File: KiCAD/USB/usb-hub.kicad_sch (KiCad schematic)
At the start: 3 parts, among them J1 Conn_01x10_Pin, J2 Conn_01x10_Pin, J3 Conn_01x04_Socket

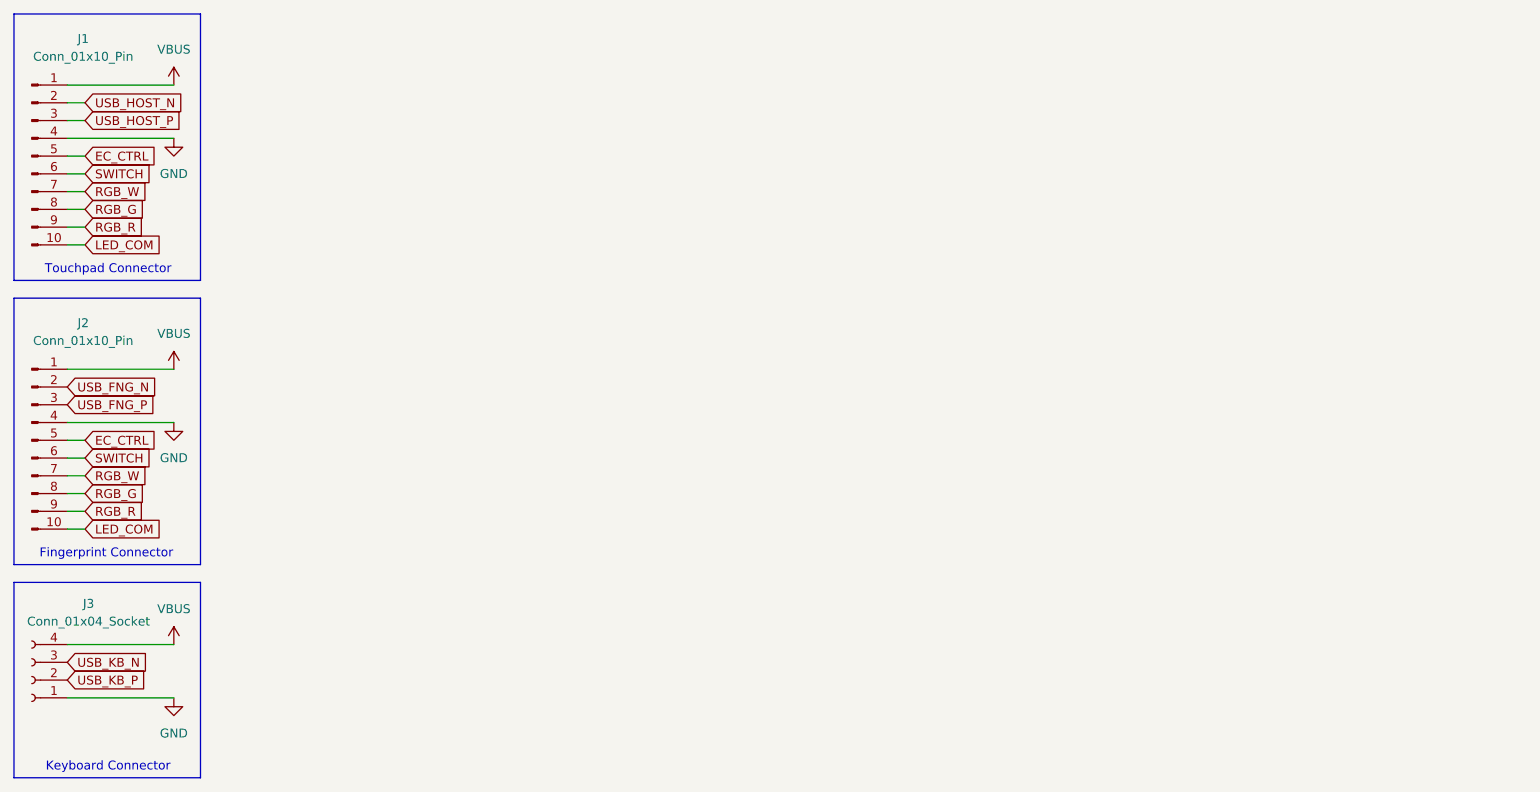
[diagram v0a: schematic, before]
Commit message: mmmm... usb hub controller...
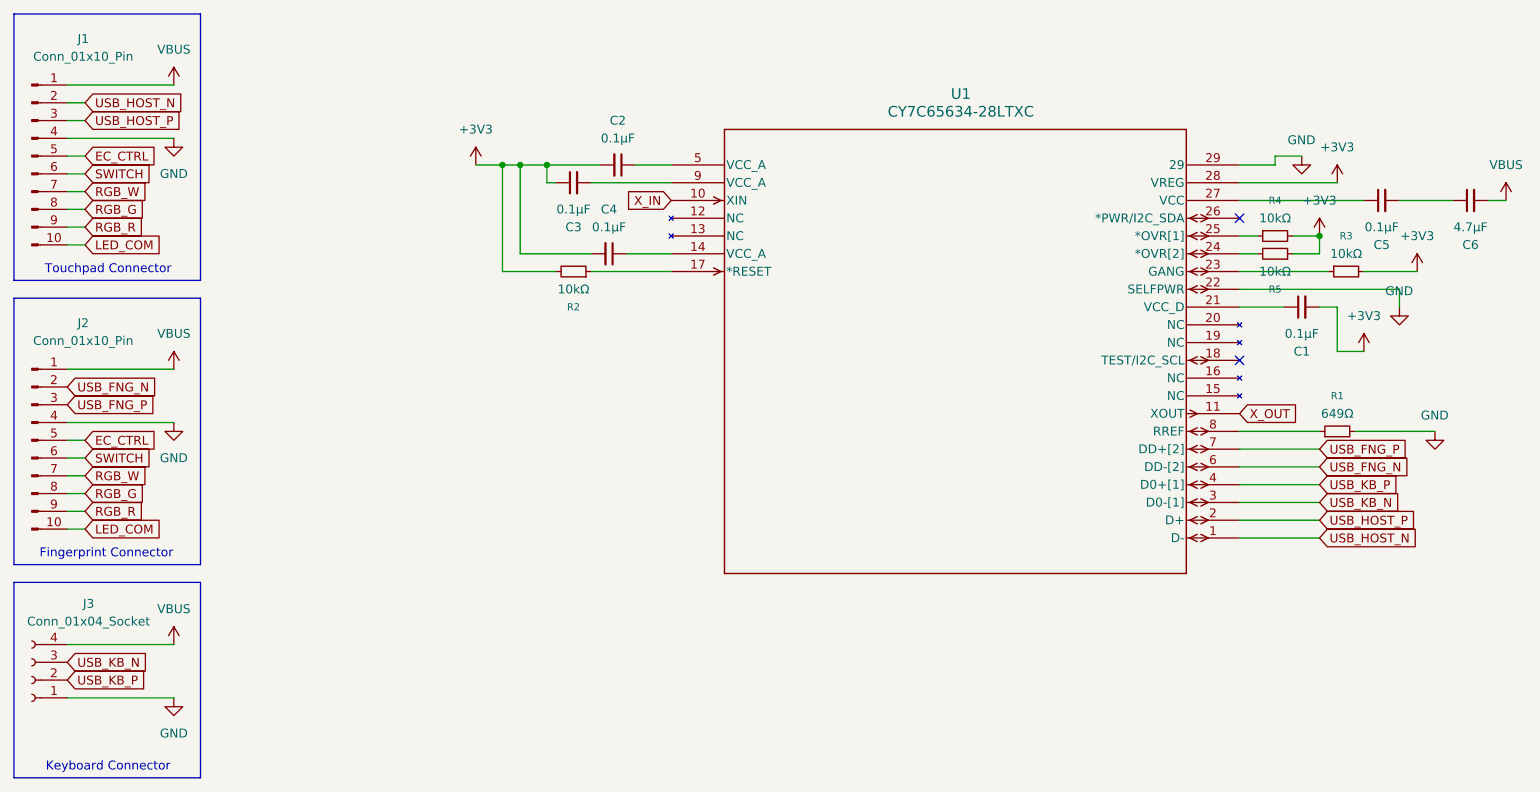
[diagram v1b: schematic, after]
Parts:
- added C1, C2, C3, C4, C5: 0.1μF, symbol Device:C_Small
- added C6: 4.7μF, symbol Device:C_Small
- added R1: 649Ω, symbol Device:R_Small
- added R2, R3, R4, R5: 10kΩ, symbol Device:R_Small
- added U1: CY7C65634-28LTXC, QFN-28, symbol 2025-09-11_12-45-01:CY7C65634-28LTXC
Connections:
- net GND: now also R1.2, U1.22 (SELFPWR), U1.29
- net USB_FNG_N: now also U1.6 (DD-[2])
- net USB_FNG_P: now also U1.7 (DD+[2])
- net USB_HOST_N: now also U1.1 (D-)
- net USB_HOST_P: now also U1.2 (D+)
- net USB_KB_N: now also U1.3 (D0-[1])
- net USB_KB_P: now also U1.4 (D0+[1])
- net VBUS: now also C6.2
- new net: R3.1, U1.23 (GANG)
- new net: C3.2, U1.9 (VCC_A)
- new net: R1.1, U1.8 (RREF)
- new net: C2.1, U1.5 (VCC_A)
- new net: R5.2, U1.24 (*OVR[2])
- new net: R4.1, U1.25 (*OVR[1])
- new net: C5.2, C6.1
- new net: C5.1, U1.27 (VCC)
- new net: R2.1, U1.17 (*RESET)
- new net: C4.1, U1.14 (VCC_A)
- new net: C1.1, U1.21 (VCC_D)
- new net +3V3: C1.2, C2.2, C3.1, C4.2, R2.2, R3.2, R4.2, R5.1, U1.28 (VREG)
- new net X_IN: U1.10 (XIN)
- new net X_OUT: U1.11 (XOUT)
- no-connect marks 0 -> 2
